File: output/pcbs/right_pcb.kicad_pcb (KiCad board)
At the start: 2 copper layers, 132 x 113 mm, 35 parts

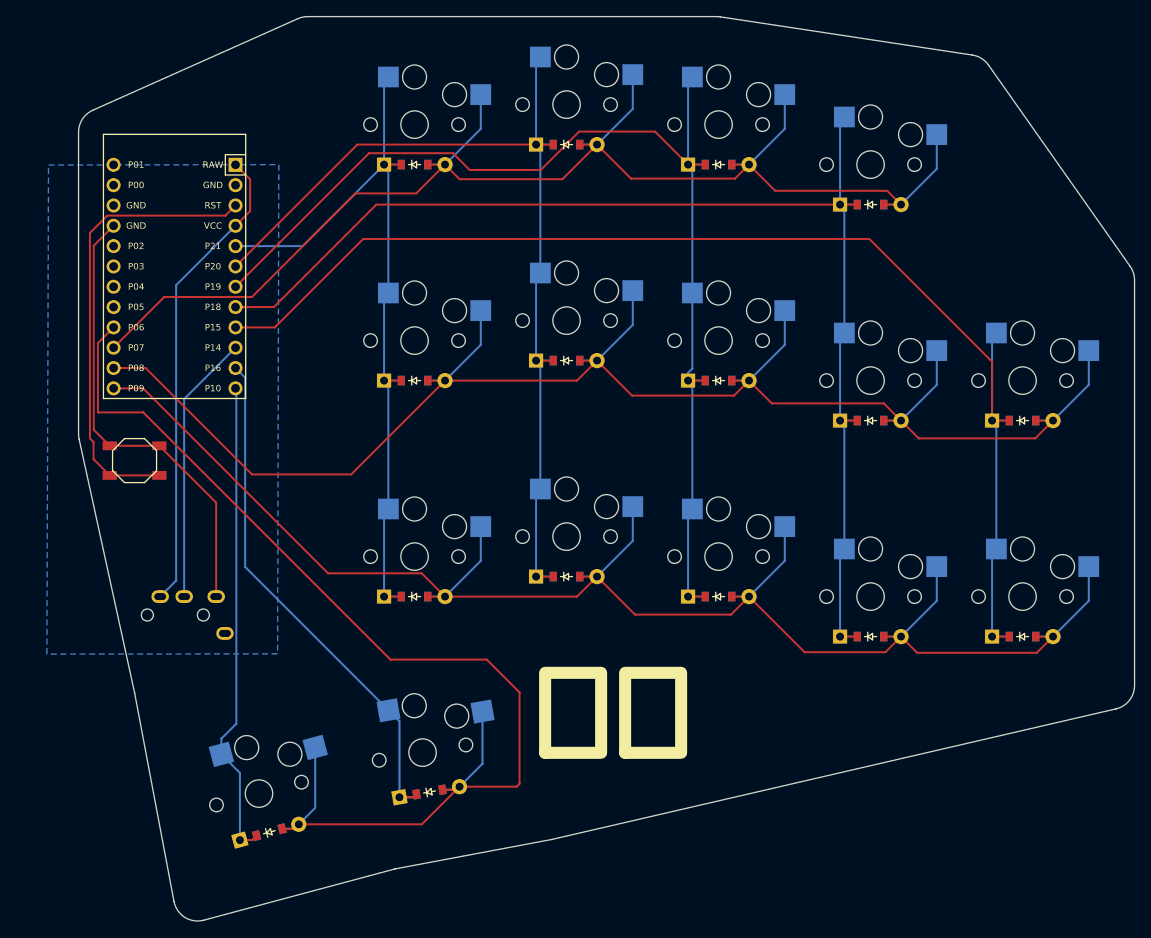
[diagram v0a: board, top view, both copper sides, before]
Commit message: fix spacing
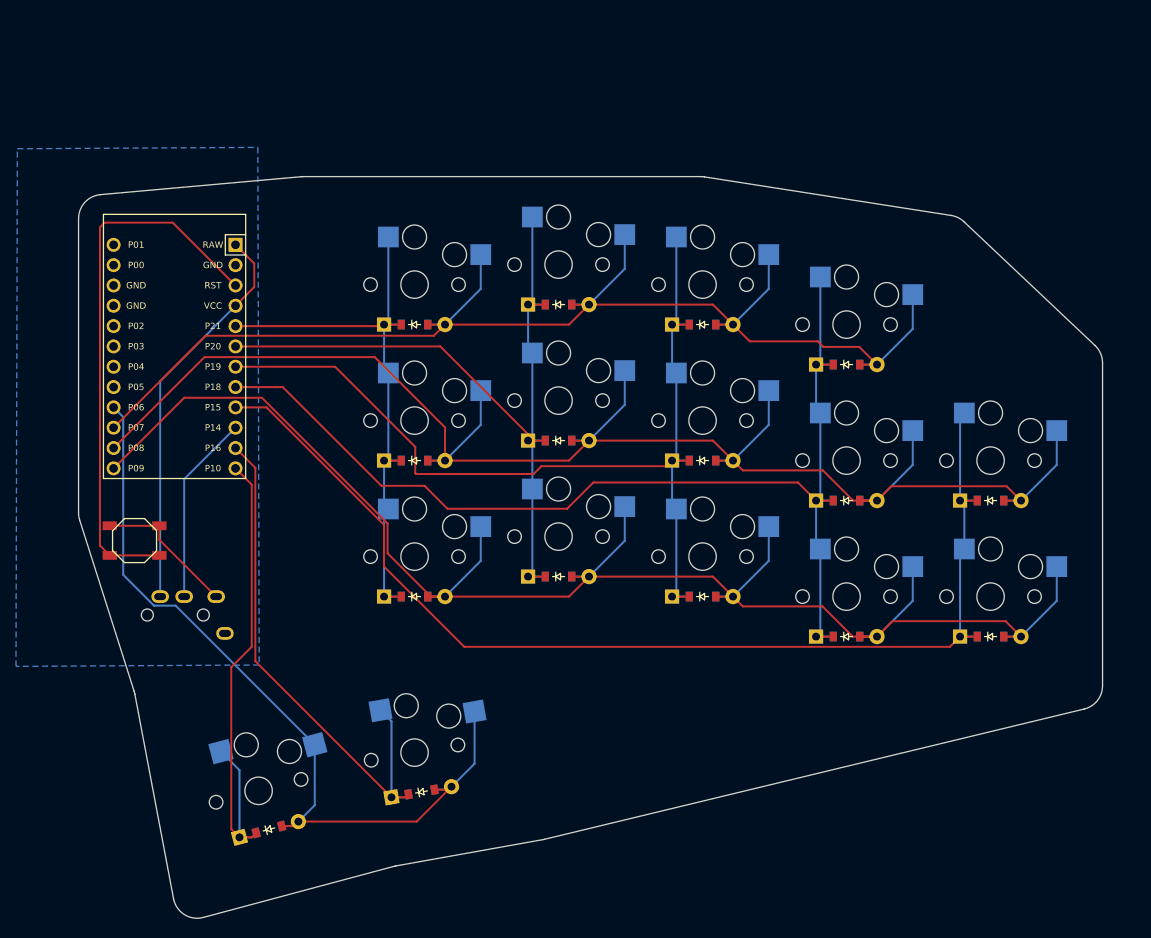
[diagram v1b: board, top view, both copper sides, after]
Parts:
- moved D12 20.2 mm to (154.0, 73.5)
- moved S12 20.2 mm to (154.0, 68.5)
- moved D9 20.1 mm to (136.0, 68.5)
- moved S9 20.1 mm to (136.0, 63.5)
- moved D6 20.0 mm to (118.0, 66.0)
- moved S6 20.0 mm to (118.0, 61.0)
- moved D3 20.0 mm to (100.0, 68.5)
- moved S3 20.0 mm to (100.0, 63.5)
- moved D14 10.8 mm to (172.0, 90.5)
- moved S14 10.8 mm to (172.0, 85.5)
- moved D11 10.4 mm to (154.0, 90.5)
- moved S11 10.4 mm to (154.0, 85.5)
- moved D8 10.2 mm to (136.0, 85.5)
- moved S8 10.2 mm to (136.0, 80.5)
- moved D5 10.0 mm to (118.0, 83.0)
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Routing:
- net R_R3: track 150.0 -> 105.4 mm
- net GND: track 57.3 -> 18.0 mm
- net R_C2: track 147.1 -> 121.8 mm
- net R_C0: track 101.8 -> 77.7 mm
- net R_C1: track 122.9 -> 100.9 mm
- net R_C3: track 159.9 -> 140.2 mm
- net R_C4: track 160.1 -> 143.8 mm
- net RST: track 57.1 -> 68.1 mm
- net R_R2: track 174.7 -> 164.6 mm
- net SERIAL: track 33.8 -> 23.8 mm
- net VCC: track 59.4 -> 49.8 mm
- net R_R1: track 209.9 -> 206.1 mm
- net R_R0: track 212.1 -> 209.9 mm
- net R_T1: track 62.9 -> 64.8 mm
- net R_T0: track 66.7 -> 67.7 mm
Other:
- board size 132 x 113 mm -> 128 x 92.7 mm
- board text removed: "安心"
